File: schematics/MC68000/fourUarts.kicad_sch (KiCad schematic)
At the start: 36 parts, among them J3 RS232_1, J4 RS232_1, J5 RS232_1, J6 RS232_1, J7 Conn_02x20_Counter_Clockwise, J8 Conn_02x04_Counter_Clockwise, J9 Conn_02x02_Counter_Clockwise, U18_C1 100nf, U18_C2 100nf, U18_C3 100nf, U18_C4 100nf, U19 UART1, U20 UART2, U21 UART3, U22 UART4, U23 74LS573, U24 74LS32, U25 74LS04, X2 16MHZ

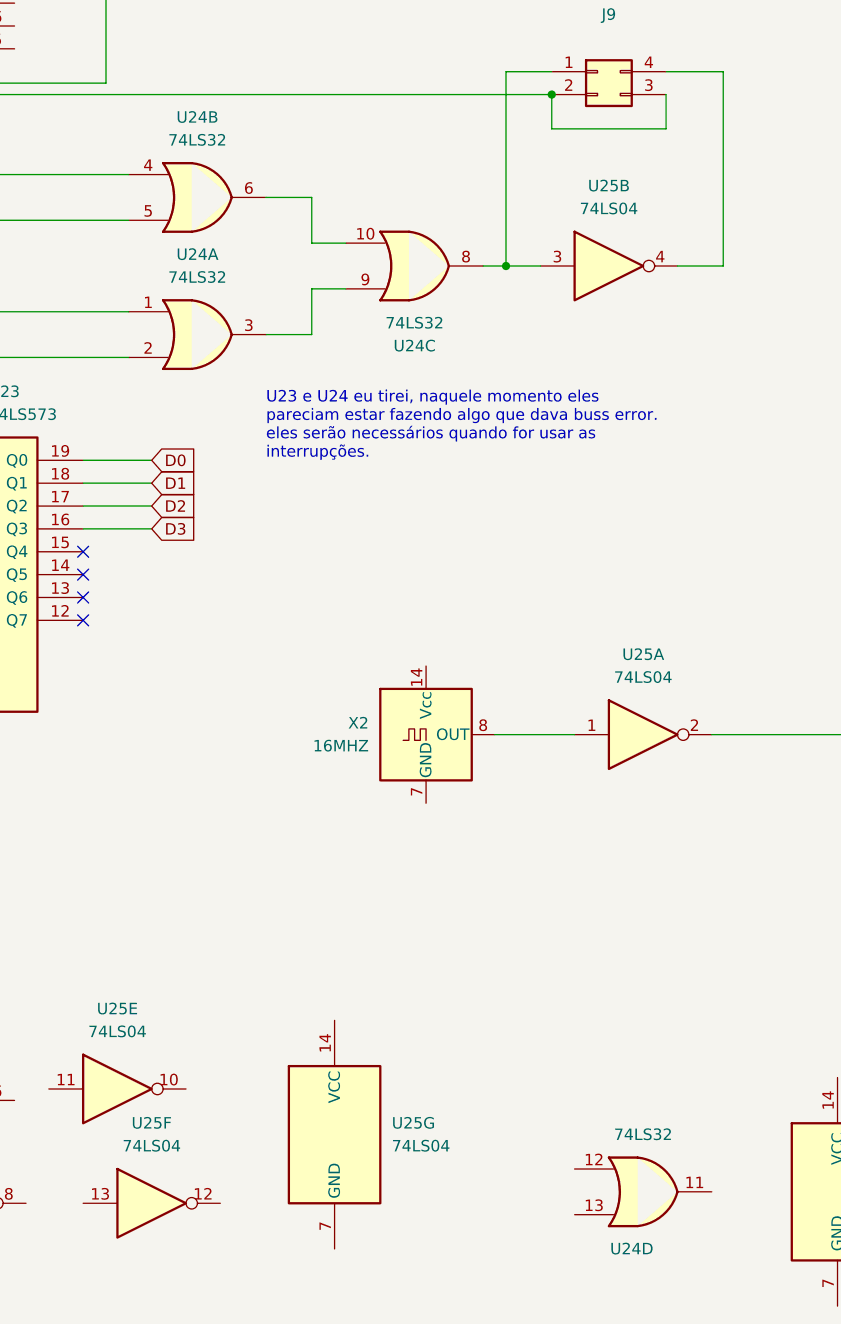
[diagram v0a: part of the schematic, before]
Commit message: updating...
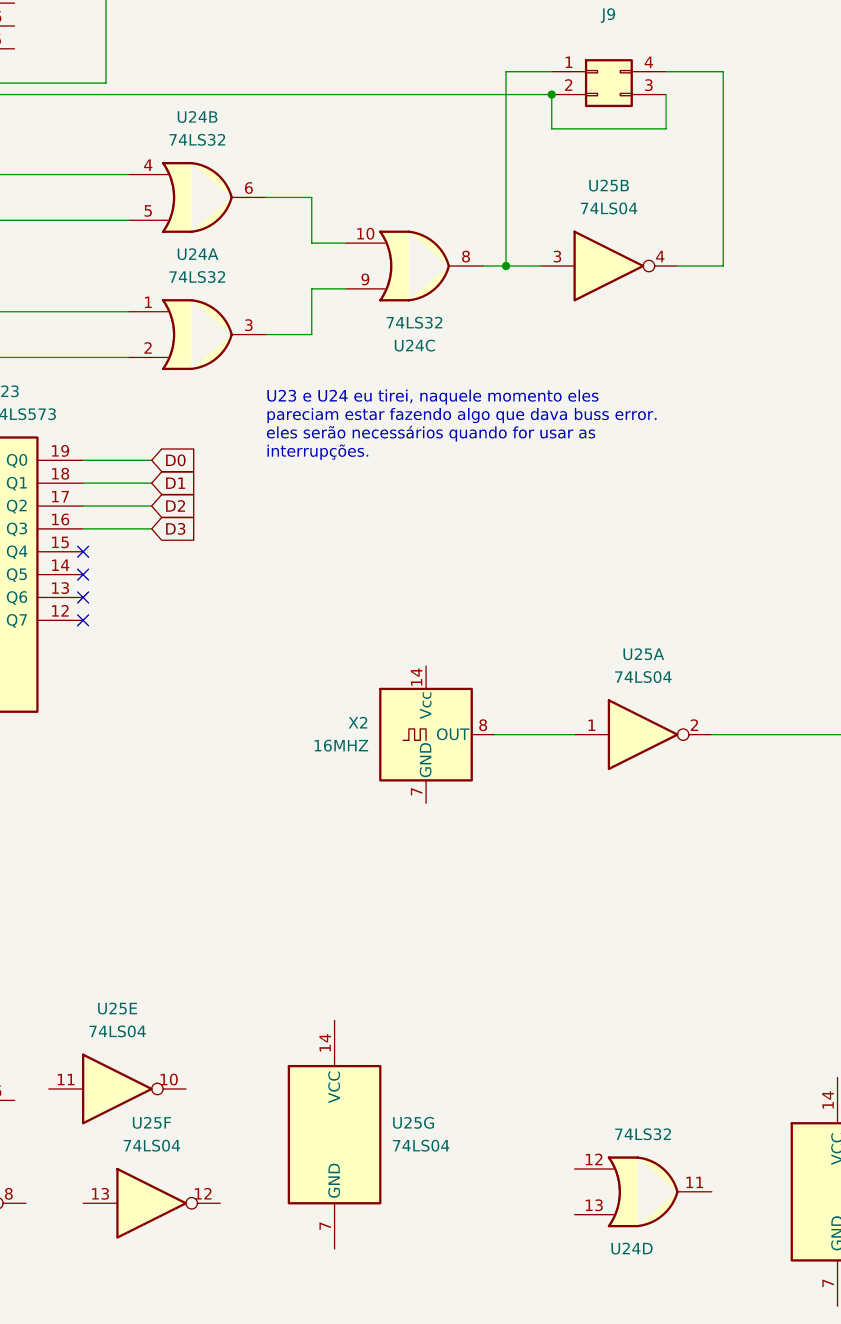
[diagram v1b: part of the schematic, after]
